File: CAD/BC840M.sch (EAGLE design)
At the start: 90 parts, among them J1 SM02B-SRSS-TB(LF)(SN), U1 TPD4S012DRYR, U2 BC840M, U3 LP5907MFX-3.3/NOPB, U4 LP5907MFX-3.3/NOPB, U5 ADS131M08IPBS, U6 BQ24072RGTR, U7 DX4R005JJ2R1800, X1 ABM3B-8.000MHZ-B2-T, X2 FC-12M

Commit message: latest
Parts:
- C15, C31: device standardparts:CAPACITOR.0201 -> standardparts:CAPACITOR.0402
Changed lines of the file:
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@@
 <grid distance="1" unitdist="mil" unit="mil" style="lines" multiple="1" display="no" altdistance="0.01" altunitdist="inch" altunit="inch"/>
 <layers>
-<layer number="1" name="Top" color="4" fill="1" visible="no" active="no"/>
-<layer number="2" name="Route2" color="16" fill="1" visible="no" active="no"/>
-<layer number="3" name="Route3" color="17" fill="1" visible="no" active="no"/>
-<layer number="4" name="Route4" color="18" fill="1" visible="no" active="no"/>
-<layer number="5" name="Route5" color="19" fill="1" visible="no" active="no"/>
-<layer number="6" name="Route6" color="25" fill="1" visible="no" active="no"/>
-<layer number="7" name="Route7" color="26" fill="1" visible="no" active="no"/>
-<layer number="8" name="Route8" color="27" fill="1" visible="no" active="no"/>
-<layer number="9" name="Route9" color="28" fill="1" visible="no" active="no"/>
-<layer number="10" name="Route10" color="29" fill="1" visible="no" active="no"/>
-<layer number="11" name="Route11" color="30" fill="1" visible="no" active="no"/>
-<layer number="12" name="Route12" color="20" fill="1" visible="no" active="no"/>
-<layer number="13" name="Route13" color="21" fill="1" visible="no" active="no"/>
-<layer number="14" name="Route14" color="22" fill="1" visible="no" active="no"/>
-<layer number="15" name="Route15" color="23" fill="1" visible="no" active="no"/>
-<layer number="16" name="Bottom" color="1" fill="1" visible="no" active="no"/>
-<layer number="17" name="Pads" color="2" fill="1" visible="no" active="no"/>
-<layer number="18" name="Vias" color="2" fill="1" visible="no" active="no"/>
-<layer number="19" name="Unrouted" color="6" fill="1" visible="no" active="no"/>
-<layer number="20" name="Dimension" color="24" fill="1" visible="no" active="no"/>
-<layer number="21" name="tPlace" color="7" fill="1" visible="no" active="no"/>
-<layer number="22" name="bPlace" color="7" fill="1" visible="no" active="no"/>
-<layer number="23" name="tOrigins" color="15" fill="1" visible="no" active="no"/>
-<layer number="24" name="bOrigins" color="15" fill="1" visible="no" active="no"/>
-<layer number="25" name="tNames" color="7" fill="1" visible="no" active="no"/>
-<layer number="26" name="bNames" color="7" fill="1" visible="no" active="no"/>
-<layer number="27" name="tValues" color="7" fill="1" visible="no" active="no"/>
-<layer number="28" name="bValues" color="7" fill="1" visible="no" active="no"/>
+<layer number="1" name="Top" color="4" fill="1" visible="yes" active="no"/>
+<layer number="2" name="Route2" color="16" fill="1" visible="yes" active="no"/>
+<layer number="3" name="Route3" color="17" fill="1" visible="yes" active="no"/>
+<layer number="4" name="Route4" color="18" fill="1" visible="yes" active="no"/>
+<layer number="5" name="Route5" color="19" fill="1" visible="yes" active="no"/>
+<layer number="6" name="Route6" color="25" fill="1" visible="yes" active="no"/>
+<layer number="7" name="Route7" color="26" fill="1" visible="yes" active="no"/>
+<layer number="8" name="Route8" color="27" fill="1" visible="yes" active="no"/>
+<layer number="9" name="Route9" color="28" fill="1" visible="yes" active="no"/>
+<layer number="10" name="Route10" color="29" fill="1" visible="yes" active="no"/>
+<layer number="11" name="Route11" color="30" fill="1" visible="yes" active="no"/>
+<layer number="12" name="Route12" color="20" fill="1" visible="yes" active="no"/>
+<layer number="13" name="Route13" color="21" fill="1" visible="yes" active="no"/>
+<layer number="14" name="Route14" color="22" fill="1" visible="yes" active="no"/>
+<layer number="15" name="Route15" color="23" fill="1" visible="yes" active="no"/>
+<layer number="16" name="Bottom" color="1" fill="1" visible="yes" active="no"/>
+<layer number="17" name="Pads" color="2" fill="1" visible="yes" active="no"/>
+<layer number="18" name="Vias" color="2" fill="1" visible="yes" active="no"/>
+<layer number="19" name="Unrouted" color="6" fill="1" visible="yes" active="no"/>
+<layer number="20" name="Dimension" color="24" fill="1" visible="yes" active="no"/>
+<layer number="21" name="tPlace" color="7" fill="1" visible="yes" active="no"/>
+<layer number="22" name="bPlace" color="7" fill="1" visible="yes" active="no"/>
+<layer number="23" name="tOrigins" color="15" fill="1" visible="yes" active="no"/>
+<layer number="24" name="bOrigins" color="15" fill="1" visible="yes" active="no"/>
+<layer number="25" name="tNames" color="7" fill="1" visible="yes" active="no"/>
+<layer number="26" name="bNames" color="7" fill="1" visible="yes" active="no"/>
+<layer number="27" name="tValues" color="7" fill="1" visible="yes" active="no"/>
+<layer number="28" name="bValues" color="7" fill="1" visible="yes" active="no"/>
 <layer number="29" name="tStop" color="7" fill="3" visible="no" active="no"/>
 <layer number="30" name="bStop" color="7" fill="6" visible="no" active="no"/>
@@
 <layer number="35" name="tGlue" color="7" fill="4" visible="no" active="no"/>
 <layer number="36" name="bGlue" color="7" fill="5" visible="no" active="no"/>
-<layer number="37" name="tTest" color="7" fill="1" visible="no" active="no"/>
-<layer number="38" name="bTest" color="7" fill="1" visible="no" active="no"/>
+<layer number="37" name="tTest" color="7" fill="1" visible="yes" active="no"/>
+<layer number="38" name="bTest" color="7" fill="1" visible="yes" active="no"/>
 <layer number="39" name="tKeepout" color="4" fill="11" visible="no" active="no"/>
 <layer number="40" name="bKeepout" color="1" fill="11" visible="no" active="no"/>
@@
 <layer number="44" name="Drills" color="7" fill="1" visible="no" active="no"/>
 <layer number="45" name="Holes" color="7" fill="1" visible="no" active="no"/>
-<layer number="46" name="Milling" color="3" fill="1" visible="no" active="no"/>
-<layer number="47" name="Measures" color="7" fill="1" visible="no" active="no"/>
-<layer number="48" name="Document" color="7" fill="1" visible="no" active="no"/>
-<layer number="49" name="Reference" color="7" fill="1" visible="no" active="no"/>
-<layer number="50" name="dxf" color="7" fill="1" visible="no" active="no"/>
-<layer number="51" name="tDocu" color="7" fill="1" visible="no" active="no"/>
-<layer number="52" name="bDocu" color="7" fill="1" visible="no" active="no"/>
-<layer number="53" name="tGND_GNDA" color="7" fill="9" visible="no" active="no"/>
-<layer number="54" name="bGND_GNDA" color="1" fill="9" visible="no" active="no"/>
-<layer number="56" name="wert" color="7" fill="1" visible="no" active="no"/>
-<layer number="57" name="tCAD" color="7" fill="1" visible="no" active="no"/>
-<layer number="58" name="bCAD" color="7" fill="1" visible="no" active="no"/>
-<layer number="59" name="tCarbon" color="7" fill="1" visible="no" active="no"/>
-<layer number="60" name="bCarbon" color="7" fill="1" visible="no" active="no"/>
+<layer number="46" name="Milling" color="3" fill="1" visible="yes" active="no"/>
+<layer number="47" name="Measures" color="7" fill="1" visible="yes" active="no"/>
+<layer number="48" name="Document" color="7" fill="1" visible="yes" active="no"/>
+<layer number="49" name="Reference" color="7" fill="1" visible="yes" active="no"/>
+<layer number="50" name="dxf" color="7" fill="1" visible="yes" active="no"/>
+<layer number="51" name="tDocu" color="7" fill="1" visible="yes" active="no"/>
+<layer number="52" name="bDocu" color="7" fill="1" visible="yes" active="no"/>
+<layer number="53" name="tGND_GNDA" color="7" fill="9" visible="yes" active="no"/>
+<layer number="54" name="bGND_GNDA" color="1" fill="9" visible="yes" active="no"/>
+<layer number="56" name="wert" color="7" fill="1" visible="yes" active="no"/>
+<layer number="57" name="tCAD" color="7" fill="1" visible="yes" active="no"/>
+<layer number="58" name="bCAD" color="7" fill="1" visible="yes" active="no"/>
+<layer number="59" name="tCarbon" color="7" fill="1" visible="yes" active="no"/>
+<layer number="60" name="bCarbon" color="7" fill="1" visible="yes" active="no"/>
 <layer number="88" name="SimResults" color="9" fill="1" visible="yes" active="yes"/>
 <layer number="89" name="SimProbes" color="9" fill="1" visible="yes" active="yes"/>
@@
 <part name="SUPPLY7" library="supply2" library_urn="urn:adsk.eagle:library:372" deviceset="GND" device=""/>
 <part name="SUPPLY11" library="supply2" library_urn="urn:adsk.eagle:library:372" deviceset="GND" device=""/>
-<part name="C15" library="standardparts" deviceset="CAPACITOR" device=".0201" value="10uF"/>
+<part name="C15" library="standardparts" deviceset="CAPACITOR" device=".0402" value="10uF"/>
 <part name="SUPPLY13" library="supply2" library_urn="urn:adsk.eagle:library:372" deviceset="GND" device=""/>
 <part name="U2" library="BC840M" deviceset="BC840M" device=""/>
@@
 <part name="SUPPLY10" library="supply2" library_urn="urn:adsk.eagle:library:372" deviceset="GND" device=""/>
 <part name="C30" library="standardparts" deviceset="CAPACITOR" device=".0201" value="0.1uF"/>
-<part name="C31" library="standardparts" deviceset="CAPACITOR" device=".0201" value="10uF"/>
+<part name="C31" library="standardparts" deviceset="CAPACITOR" device=".0402" value="10uF"/>
 </parts>
 <sheets>

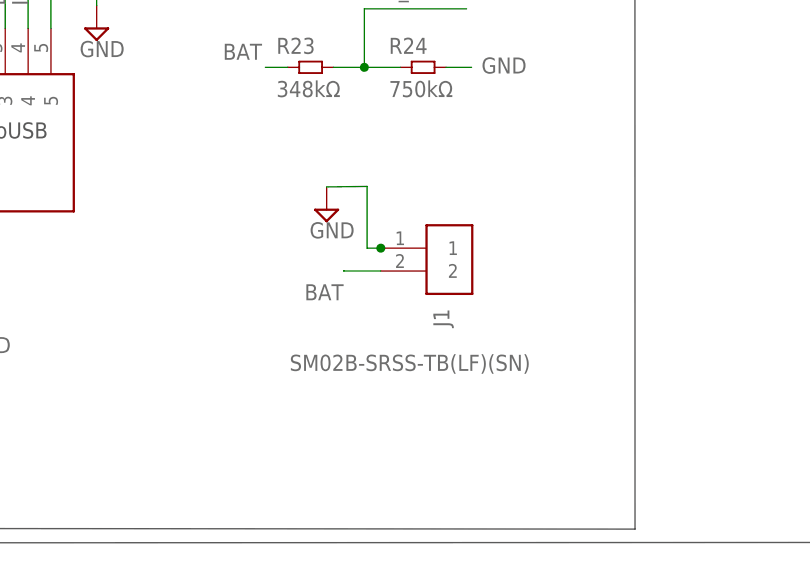
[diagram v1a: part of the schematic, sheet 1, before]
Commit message: edits and CAM
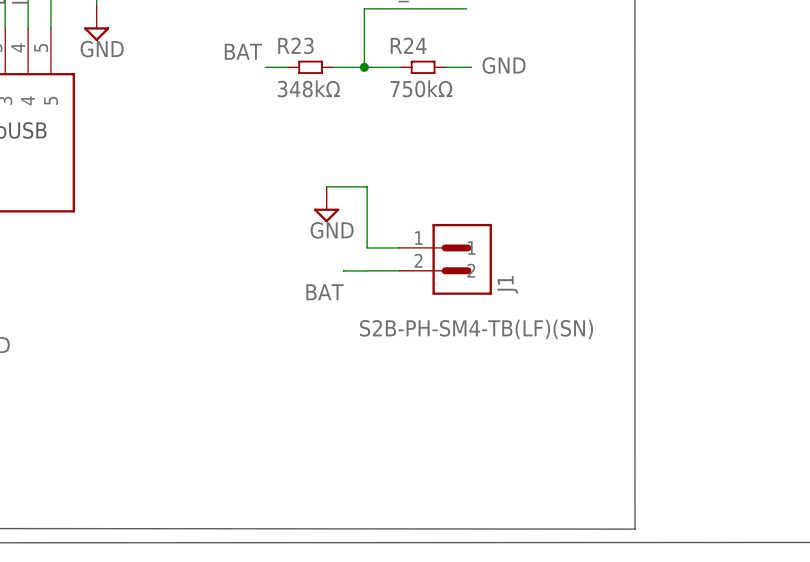
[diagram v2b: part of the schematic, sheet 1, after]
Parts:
- J1: value SM02B-SRSS-TB(LF)(SN) -> S2B-PH-SM4-TB(LF)(SN); device SM02B-SRSS-TB_LF__SN_:SM02B-SRSS-TB(LF)(SN) -> S2B-PH-SM4-TB_LF__SN_:S2B-PH-SM4-TB(LF)(SN)

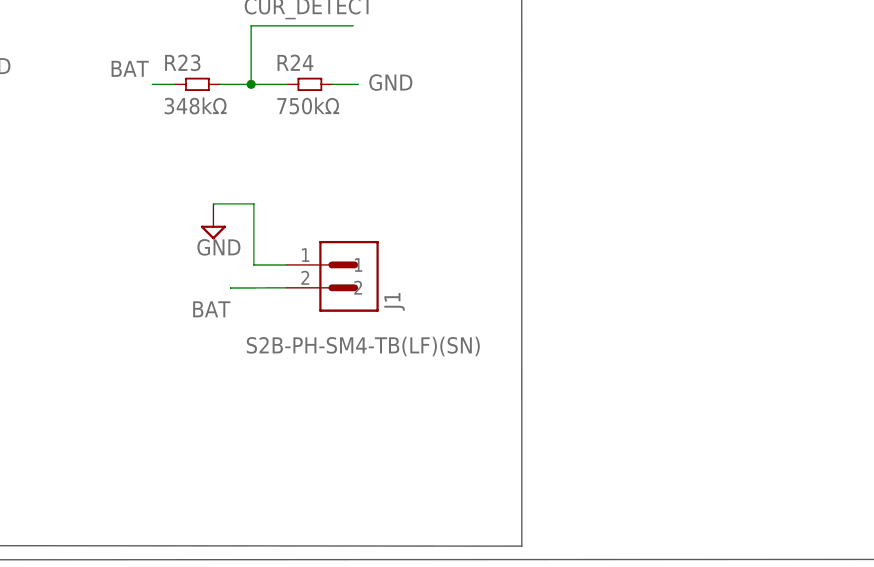
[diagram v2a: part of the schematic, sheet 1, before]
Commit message: fix
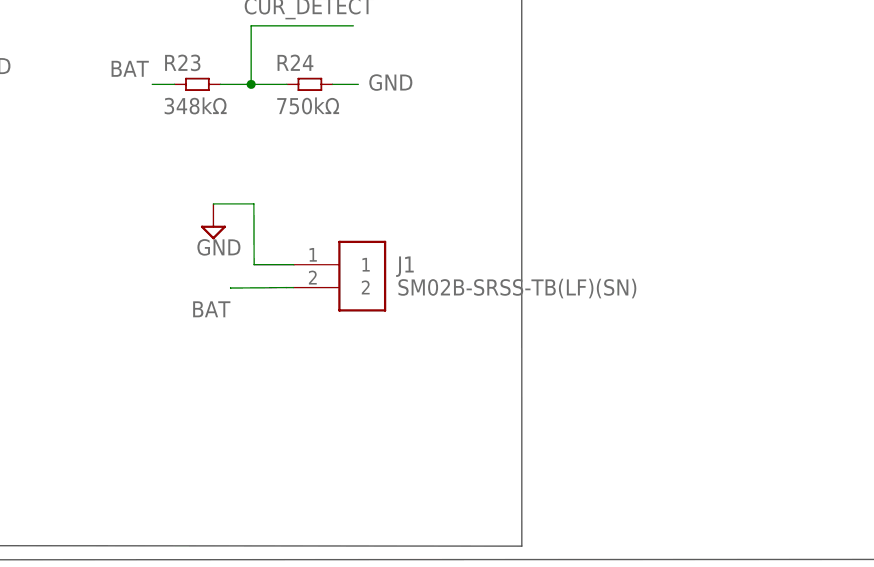
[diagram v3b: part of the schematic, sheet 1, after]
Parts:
- J1: value S2B-PH-SM4-TB(LF)(SN) -> SM02B-SRSS-TB(LF)(SN); device S2B-PH-SM4-TB_LF__SN_:S2B-PH-SM4-TB(LF)(SN) -> SM02B-SRSS-TB_LF__SN_:SM02B-SRSS-TB(LF)(SN)
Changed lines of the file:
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@@
 <part name="U2" library="BC840M" deviceset="BC840M" device=""/>
 <part name="U6" library="BQ24072RGTR" deviceset="BQ24072RGTR" device=""/>
-<part name="J1" library="S2B-PH-SM4-TB_LF__SN_" deviceset="S2B-PH-SM4-TB(LF)(SN)" device=""/>
 <part name="JP1" library="pinhead+" deviceset="PINHD-2X8" device="SMT"/>
 <part name="JP2" library="pinhead+" deviceset="PINHD-2X10" device="SMT"/>
@@
 <part name="C30" library="standardparts" deviceset="CAPACITOR" device=".0201" value="0.1uF"/>
 <part name="C31" library="standardparts" deviceset="CAPACITOR" device=".0402" value="10uF"/>
+<part name="J1" library="SM02B-SRSS-TB_LF__SN_" deviceset="SM02B-SRSS-TB(LF)(SN)" device=""/>
 </parts>
 <sheets>
@@
 <attribute name="VALUE" x="55.7022" y="84.265" size="2.0828" layer="96" ratio="10" rot="SR0"/>
 </instance>
-<instance part="J1" gate="G$1" x="89.1286" y="37.9476" smashed="yes">
-<attribute name="NAME" x="95.85583125" y="34.252" size="1.78541875" layer="95" rot="R90" align="center-left"/>
-<attribute name="VALUE" x="105.7556" y="30.283959375" size="1.784809375" layer="96" rot="R180" align="center-left"/>
-</instance>
 <instance part="JP1" gate="A" x="328.5236" y="120.3706" smashed="yes">
 <attribute name="NAME" x="322.1736" y="131.1656" size="1.778" layer="95"/>
@@
 <attribute name="NAME" x="23.5204" y="75.0824" size="1.016" layer="95" rot="MR0"/>
 <attribute name="VALUE" x="23.5204" y="77.6224" size="1.016" layer="96" rot="R180"/>
+</instance>
+<instance part="J1" gate="G$1" x="84.8868" y="34.163" smashed="yes">
+<attribute name="NAME" x="96.3804" y="39.27216875" size="1.78541875" layer="95" align="center-left"/>
+<attribute name="VALUE" x="96.3776" y="36.721240625" size="1.784809375" layer="96" align="center-left"/>
 </instance>
 </instances>
@@
 <junction x="37.719" y="35.9156"/>
 <pinref part="SUPPLY13" gate="GND" pin="GND"/>
-</segment>
-<segment>
-<wire x1="84.0486" y1="39.2176" x2="80.4672" y2="39.2176" width="0.1524" layer="91"/>
-<wire x1="80.4672" y1="39.2176" x2="80.4672" y2="45.9994" width="0.1524" layer="91"/>
-<pinref part="SUPPLY7" gate="GND" pin="GND"/>
-<wire x1="80.4672" y1="45.9994" x2="75.9714" y2="45.9994" width="0.1524" layer="91"/>
-<pinref part="J1" gate="G$1" pin="1"/>
 </segment>
 <segment>
@@
 <label x="22.7076" y="68.6562" size="1.778" layer="95"/>
 </segment>
+<segment>
+<pinref part="J1" gate="G$1" pin="1"/>
+<wire x1="84.8868" y1="39.243" x2="80.4926" y2="39.243" width="0.1524" layer="91"/>
+<wire x1="80.4926" y1="39.243" x2="80.4672" y2="45.9994" width="0.1524" layer="91"/>
+<pinref part="SUPPLY7" gate="GND" pin="GND"/>
+<wire x1="80.4672" y1="45.9994" x2="75.9714" y2="45.9994" width="0.1524" layer="91"/>
+</segment>
 </net>
 <net name="CLKIN" class="0">
@@
 </segment>
 <segment>
-<pinref part="J1" gate="G$1" pin="2"/>
-<wire x1="84.0486" y1="36.6776" x2="77.8764" y2="36.6522" width="0.1524" layer="91"/>
+<wire x1="84.0486" y1="36.703" x2="77.8764" y2="36.6522" width="0.1524" layer="91"/>
 <wire x1="77.8764" y1="36.6522" x2="77.8764" y2="36.6776" width="0.1524" layer="91"/>
 <label x="77.851" y="35.179" size="1.778" layer="95" rot="R180"/>
-</segment>
-<segment>
+<pinref part="J1" gate="G$1" pin="2"/>
+<wire x1="84.8868" y1="36.703" x2="84.0486" y2="36.703" width="0.1524" layer="91"/>
+</segment>
+<segment>
